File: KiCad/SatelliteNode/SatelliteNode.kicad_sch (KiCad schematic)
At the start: 26 parts, among them J1 12V_Connector, J2 Isolated_RS485, J3 Conn_01x04, J4 Conn_01x04, J5 Conn_01x04, J6 Conn_01x04, J7 Conn_01x04, J8 Conn_01x04, U2 SSD1306, U3 XIAO-ESP32-C6, U4 MCP23017_SP, U5 74HC14, U6 BP5293-50

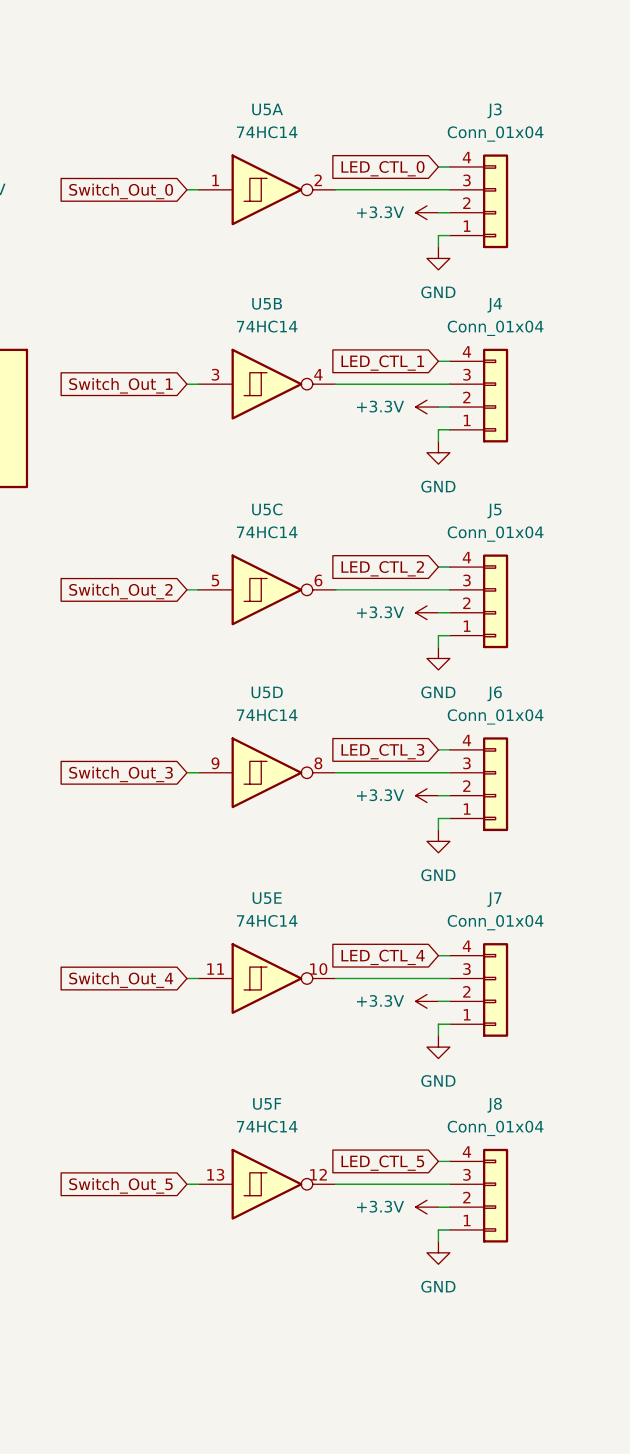
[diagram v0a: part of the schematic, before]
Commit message: Build-2 を発行
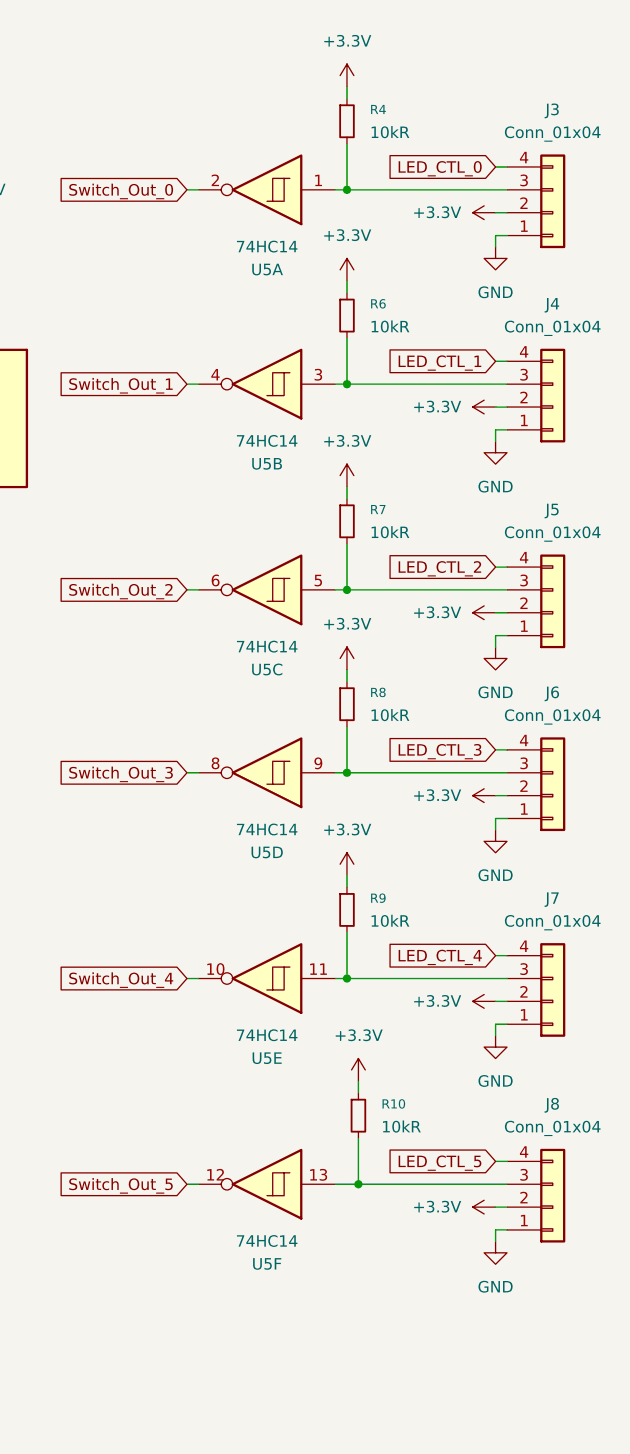
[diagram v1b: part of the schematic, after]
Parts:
- added R10, R4, R6, R7, R8, R9: 10kR, Resistor_SMD:R_0603_1608Metric, symbol Device:R_Small
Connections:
- net +3.3V: now also R10.1, R4.1, R6.1, R7.1, R8.1, R9.1
- net Switch_Out_0: now also U5.2; no longer U5.1
- net Switch_Out_1: now also U5.4; no longer U5.3
- net Switch_Out_2: now also U5.6; no longer U5.5
- net Switch_Out_3: now also U5.8; no longer U5.9
- net Switch_Out_4: now also U5.10; no longer U5.11
- net Switch_Out_5: now also U5.12; no longer U5.13
- net at J6.3 (Pin_3): now also U5.9, R8.2; no longer U5.8
- net at J7.3 (Pin_3): now also U5.11, R9.2; no longer U5.10
- net at J8.3 (Pin_3): now also U5.13, R10.2; no longer U5.12
- net at J5.3 (Pin_3): now also U5.5, R7.2; no longer U5.6
- net at J3.3 (Pin_3): now also U5.1, R4.2; no longer U5.2
- net at J4.3 (Pin_3): now also U5.3, R6.2; no longer U5.4
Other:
- moved on the sheet: J3, J4, J5, J6, J7, J8, U5A, U5B, U5C, U5D, U5E, U5F
